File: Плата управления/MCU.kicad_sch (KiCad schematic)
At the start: 39 parts, among them U7 ASEMB-10, U8 STM32F407VETx

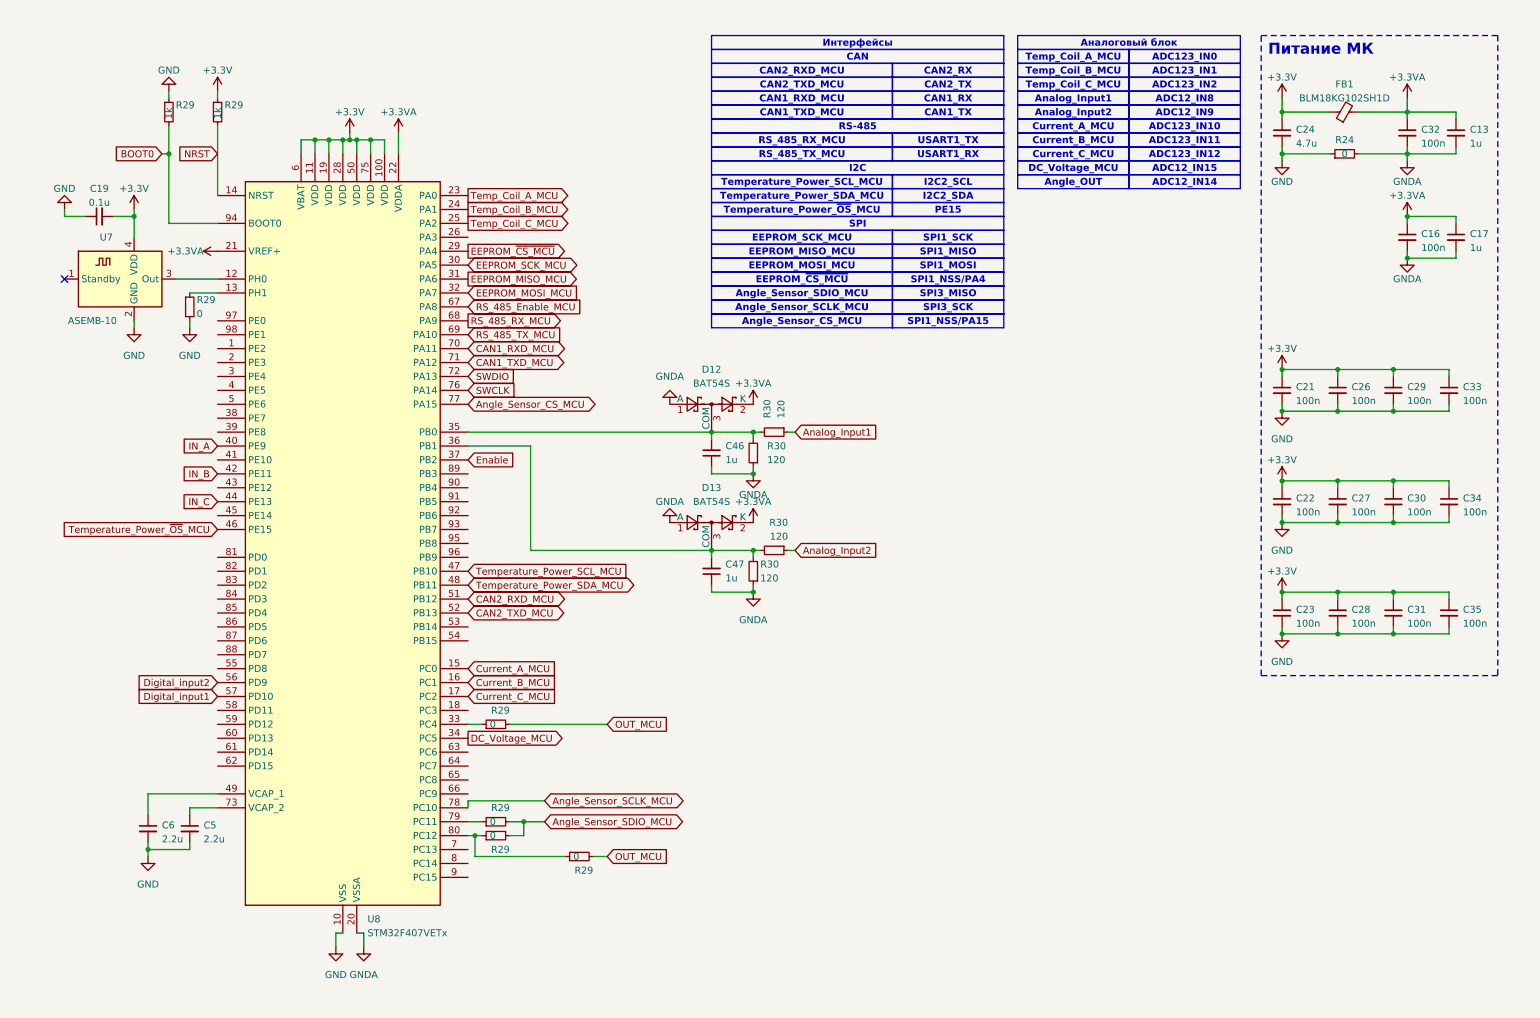
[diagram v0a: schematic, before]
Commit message: Добавил документы
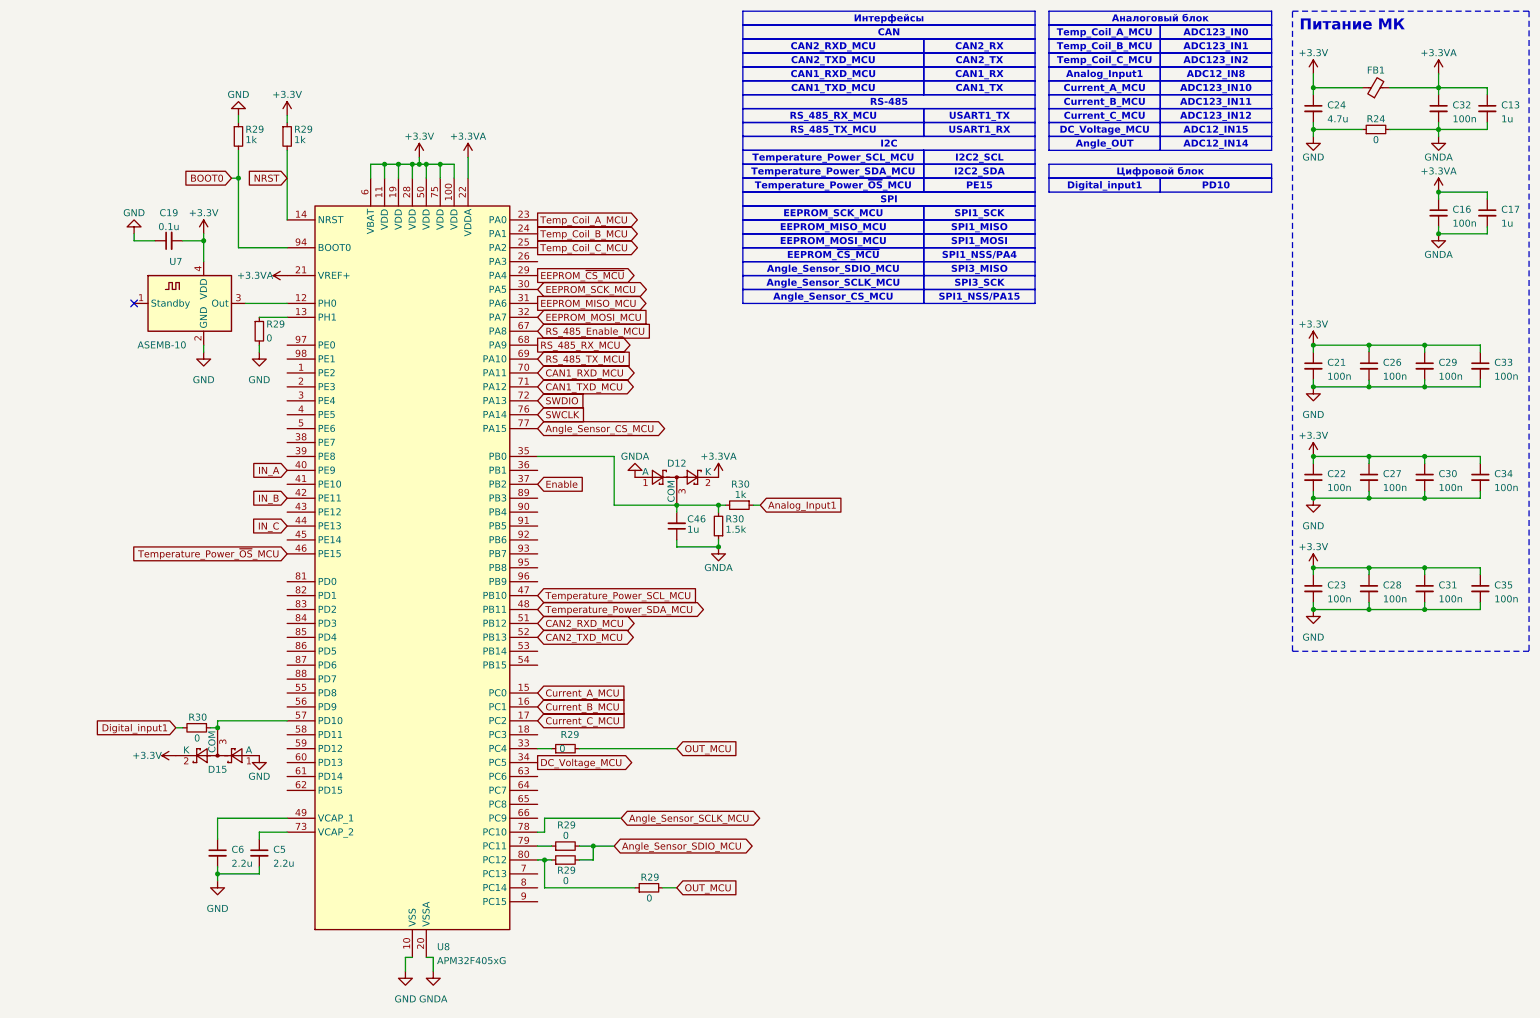
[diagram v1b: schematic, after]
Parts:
- removed C47: 1u, Capacitor_SMD:C_0603_1608Metric_Pad1.08x0.95mm_HandSolder, symbol Device:C_Small
- removed D13: BAT54S, Package_TO_SOT_SMD:SOT-23, symbol Diode:BAT54S
- removed R30 (x2): 120, Resistor_SMD:R_0603_1608Metric_Pad0.98x0.95mm_HandSolder, symbol Device:R_Small
- added D15: BAT54S, Package_TO_SOT_SMD:SOT-23, symbol Diode:BAT54S
- added R30: 0, Resistor_SMD:R_0603_1608Metric_Pad0.98x0.95mm_HandSolder, symbol Device:R_Small
- R30: value 120 -> 1.5k
- R30: value 120 -> 1k
- U8: value STM32F407VETx -> APM32F405xG
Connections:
- net +3.3V: now also D15.2 (K)
- net Digital_input1: now also R30.2; no longer U8.57 (PD10)
- net GND: now also D15.1 (A)
- net Digital_input2: no longer names the net of U8.56 (PD9)
- new net: D15.3 (COM), R30.1, U8.57 (PD10)
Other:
- moved on the sheet: C13, C16, C17, C19, C21, C22, C23, C24, C26, C27, C28, C29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
